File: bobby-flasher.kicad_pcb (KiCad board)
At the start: 2 copper layers, 17.4 x 29.4 mm, 28 parts, among them J1 Conn_01x03, J2 Conn_01x06, J3 Flash, Q1 SS8050_C2150, Q2 SS8050_C2150, U1 CH343G, U2 AMS1117-3.3

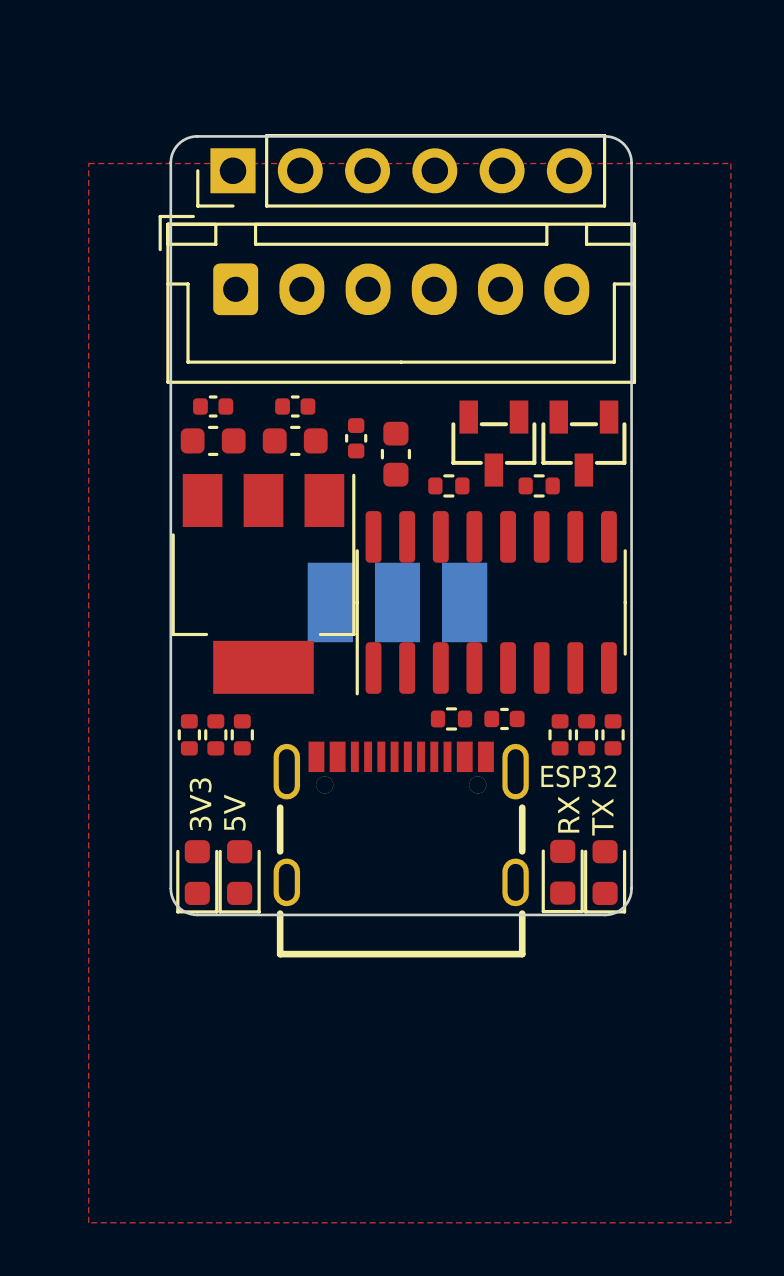
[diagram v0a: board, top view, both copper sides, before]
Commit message: Updated pcb
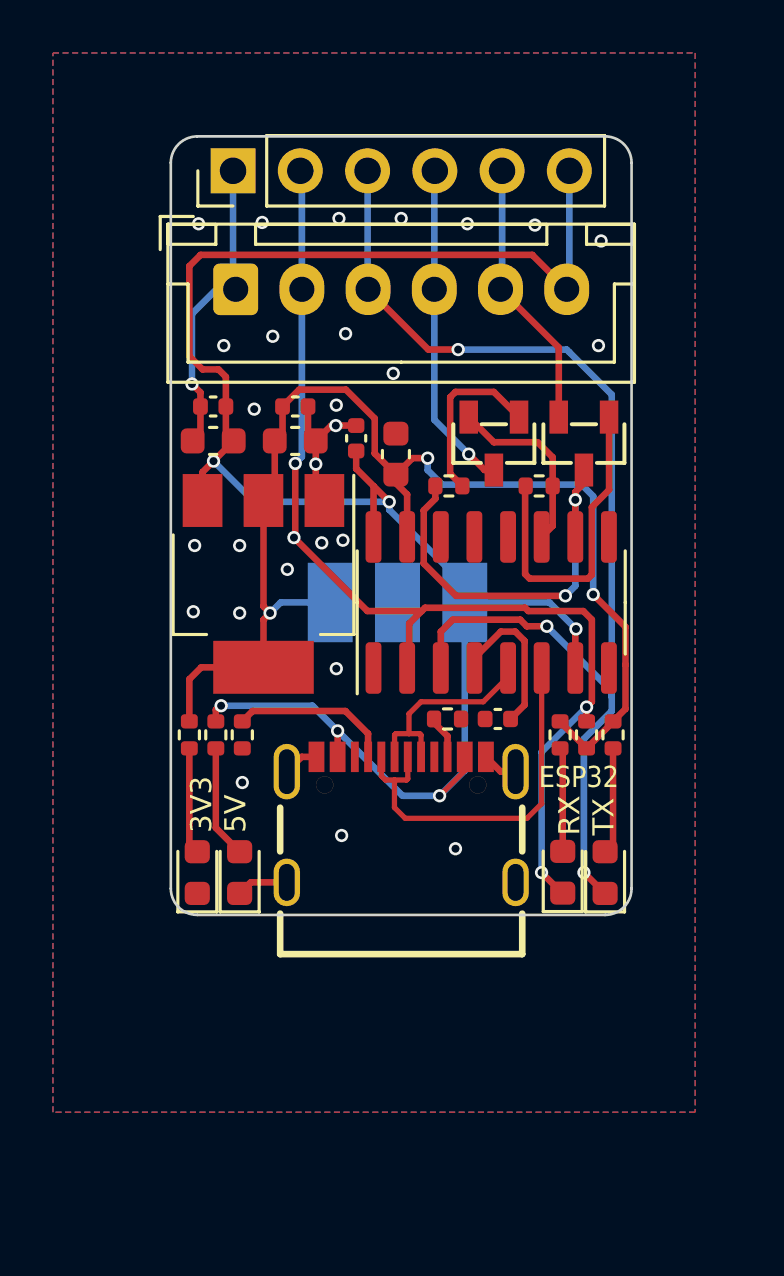
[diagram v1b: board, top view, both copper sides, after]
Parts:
- moved C3 0.25 mm to (3.65, 73.6)
- moved R3 0.15 mm to (1.75, 73.6)
- turned R6 to -90 degrees
- turned R7 to -90 degrees
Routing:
- net +5V: track 0.00 -> 73.5 mm, vias 0 -> 6
- net +3V3: track 0.00 -> 47.2 mm, vias 0 -> 3
- net ESP_TX: track 0.00 -> 44.3 mm, vias 0 -> 3
- net ESP_RX: track 0.00 -> 41.0 mm, vias 0 -> 4
- net GND: track 0.00 -> 21.8 mm, vias 0 -> 28
- net DTR: track 0.00 -> 15.4 mm, vias 0 -> 2
- net USB_DN: track 0.00 -> 14.7 mm
- net EN: track 0.00 -> 12.4 mm, vias 0 -> 1
- net Net-(Q2-Pad1): track 0.00 -> 12.2 mm
- net IO0: track 0.00 -> 10.2 mm
- net USB_DP: track 0.00 -> 8.10 mm
- net RTS: track 0.00 -> 6.98 mm
- net Net-(Q1-Pad1): track 0.00 -> 6.62 mm
- net Net-(R1-Pad1): track 0.00 -> 6.14 mm
- net Net-(C3-Pad2): track 0.00 -> 6.00 mm
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- added copper zone on B.Cu, net GND
